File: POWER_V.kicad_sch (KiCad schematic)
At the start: 23 parts, among them CN1 XT30PW-M, CN2 XT30PW-M, SW3 SWITCH_BLACK, SW4 SWITCH_BLACK, U7 XL4005E1, U8 XC6220B331MR

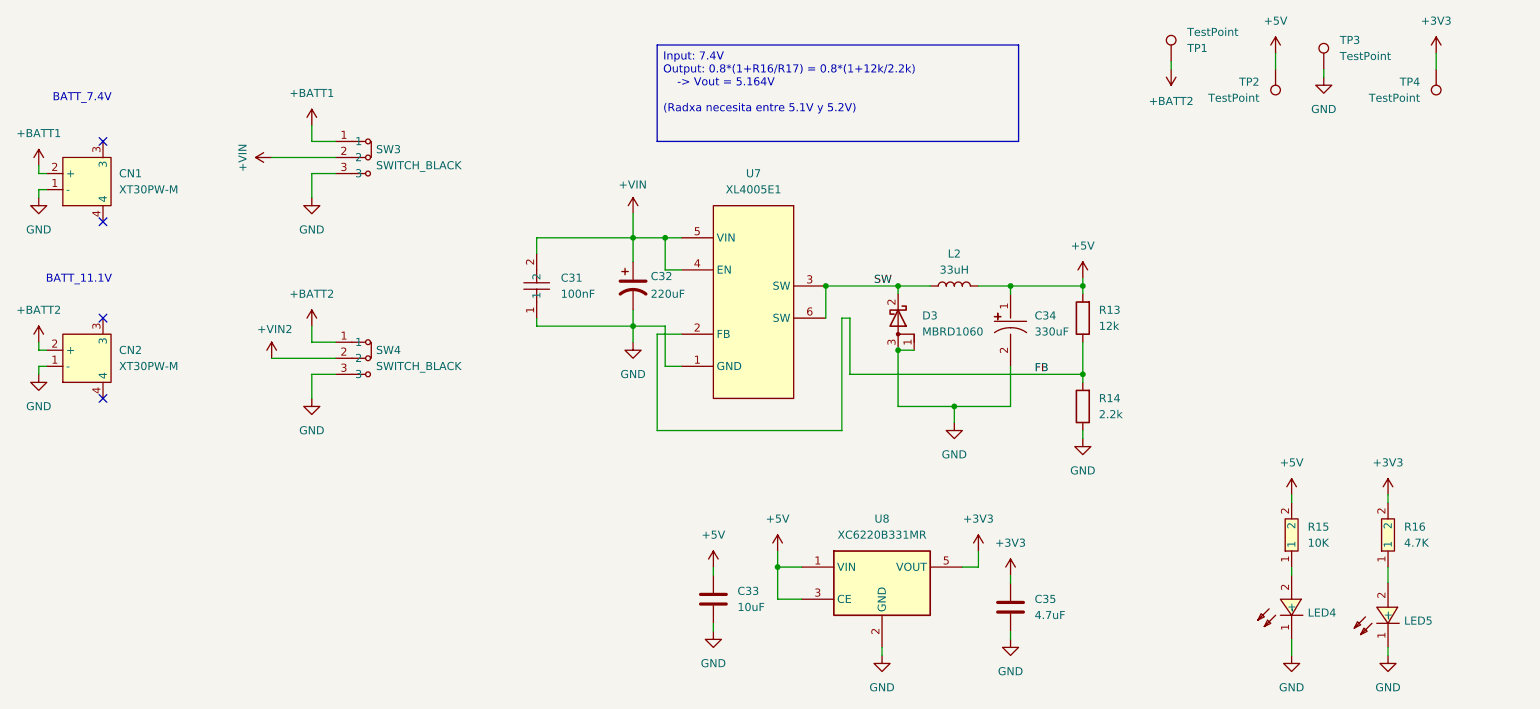
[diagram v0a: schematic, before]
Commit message: Todo antes de PCB
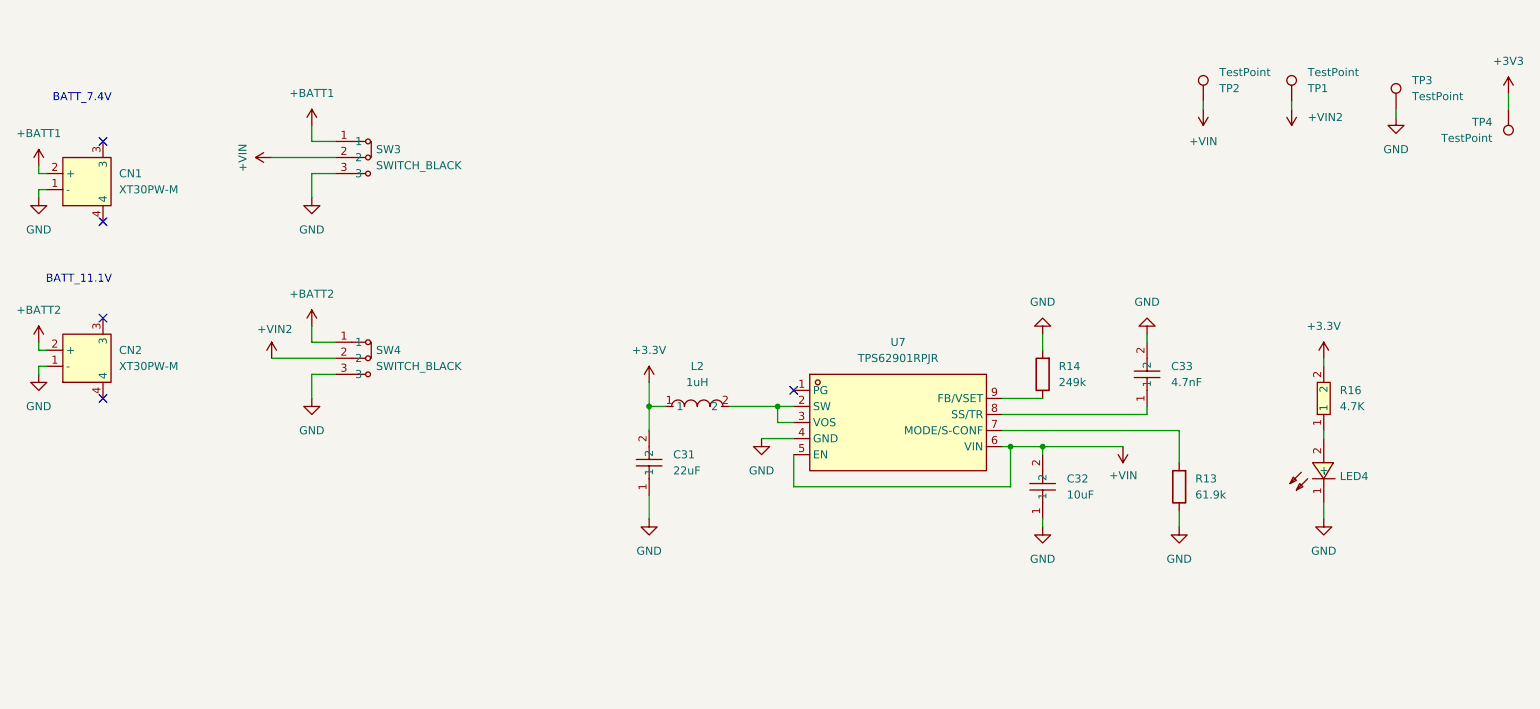
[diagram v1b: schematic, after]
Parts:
- removed C32: 220uF, ARLISS-footprints:CAP-TH_BD8.0-P3.50-D0.6-FD, symbol Device:C_Polarized_US
- removed C33: 10uF, Capacitor_SMD:C_0603_1608Metric_Pad1.08x0.95mm_HandSolder, symbol Device:C
- removed C34: 330uF, ARLISS-footprints:CAP-TH_BD10.0-P5.00-D1.0-FD, symbol CANSAT_STM32_symbols:ECR1EPT331MLL100012
- removed C35: 4.7uF, Capacitor_SMD:C_0603_1608Metric_Pad1.08x0.95mm_HandSolder, symbol Device:C
- removed D3: MBRD1060, Package_TO_SOT_SMD:TO-252-2, symbol Device:D_Schottky_AKA
- removed L2: 33uH, Inductor_SMD:L_APV_APH0850, symbol Device:L
- removed LED5: (no value), Diode_SMD:D_0603_1608Metric_Pad1.05x0.95mm_HandSolder, symbol CANSAT_STM32_symbols:D-G060306G1-KS2
- removed R15: 10K, Resistor_SMD:R_0603_1608Metric_Pad0.98x0.95mm_HandSolder, symbol CANSAT_STM32_symbols:RC0603FR-7W10KL
- removed U7: XL4005E1, ARLISS-footprints:TO-263-5_L10.2-W9.2-P1.70-TL, symbol CANSAT_STM32_symbols:XL4005E1
- removed U8: XC6220B331MR, Package_TO_SOT_SMD:SOT-23-5, symbol Regulator_Linear:XC6220B331MR
- added C32: 10uF, Capacitor_SMD:C_0805_2012Metric_Pad1.18x1.45mm_HandSolder, symbol CANSAT_STM32_symbols:TCC0402X7R104J500AT
- added C33: 4.7nF, Capacitor_SMD:C_0805_2012Metric_Pad1.18x1.45mm_HandSolder, symbol CANSAT_STM32_symbols:TCC0402X7R104J500AT
- added L2: 1uH, ARLISS-footprints:IND-SMD_L4.0-W4.0_XAL4030-332MEC, symbol CANSAT_STM32_symbols:XGL4020-102MEC
- added U7: TPS62901RPJR, ARLISS-footprints:VQFN-HR-9_L2.0-W1.5-P0.50-BL_TI_RPJ, symbol CANSAT_STM32_symbols:TPS62901RPJR
- C31: value 100nF -> 22uF; footprint Capacitor_SMD:C_0603_1608Metric_Pad1.08x0.95mm_HandSolder -> Capacitor_SMD:C_0805_2012Metric_Pad1.18x1.45mm_HandSolder; LCSC Part C5448844 -> C258782; MPN TCC0402X7R104J500AT -> GRM21BC81C226ME44L
- R13: value 12k -> 61.9k; LCSC C114659 -> C23091; Link https://www.lcsc.com/product-detail/C114659.html -> https://www.lcsc.com/datasheet/C23091.pdf?spm=wm.sxq.inf.gg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
- R14: value 2.2k -> 249k; LCSC C114662 -> C54531323; Link https://www.lcsc.com/product-detail/C114662.html -> https://www.lcsc.com/datasheet/C54531323.pdf?spm=wm.sxq.inf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
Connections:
- net FB is gone; now on net GND: R13.1, R14.2
- net +3V3: no longer R16.2
- net +BATT2: no longer TP1.1
- net +VIN: now also TP2.1, C32.2, U7.5 (EN), U7.6 (VIN); no longer C31.2
- net +VIN2: now also TP1.1
- net GND: now also C32.1, C33.2, U7.4 (GND); no longer R14.1
- net at LED4.2 (+): now also R16.1
- net +5V: no longer names the net of R13.2
- net +5V: now also U7.7 (MODE/S-CONF); no longer TP2.1
- new net: R14.1, U7.9 (FB/VSET)
- new net: L2.2, U7.2 (SW), U7.3 (VOS)
- new net: C33.1, U7.8 (SS/TR)
- new net +3.3V: C31.2, L2.1, R16.2
- no-connect marks 4 -> 5
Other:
- moved on the sheet: C31, LED4, R13, TP1, TP3, TP4
